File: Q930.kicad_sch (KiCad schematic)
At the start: 2 parts, among them U1 MW-R-WX

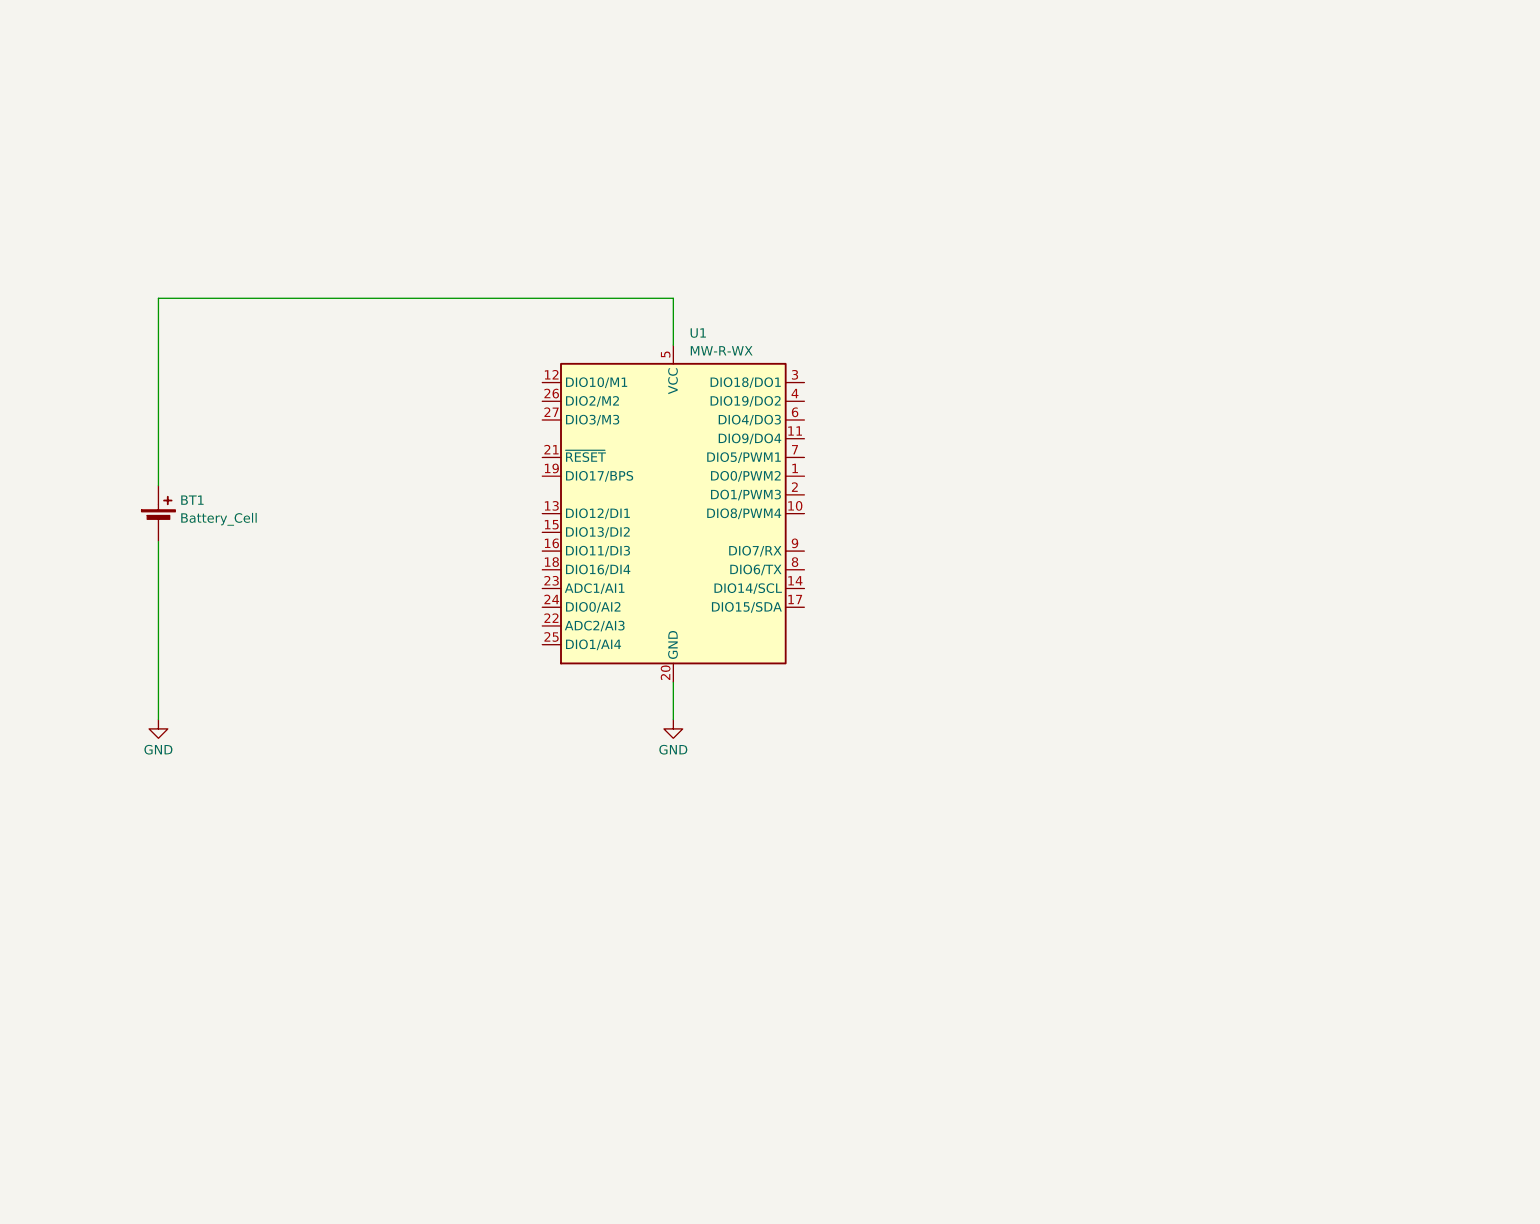
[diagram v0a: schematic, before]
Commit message: continue
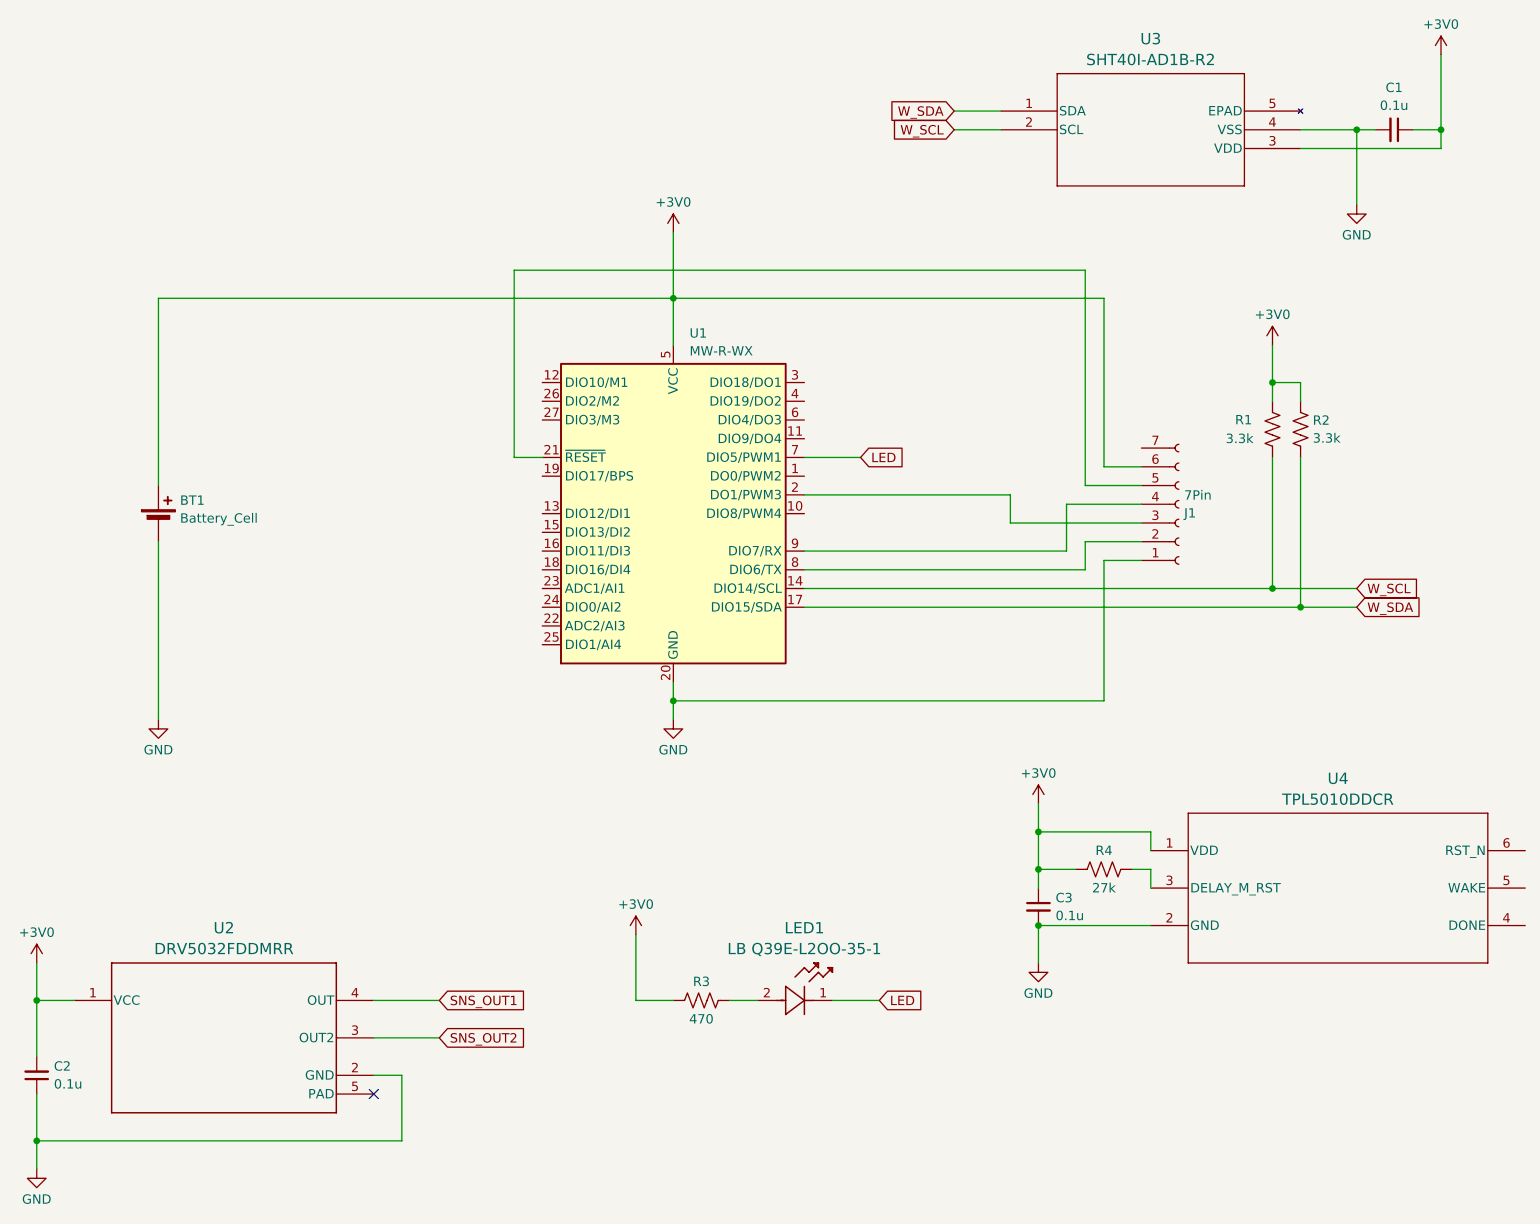
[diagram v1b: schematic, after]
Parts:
- added C1, C2, C3: 0.1u, symbol Device:C_Small
- added J1: 7Pin, symbol Connector:Conn_01x07_Socket
- added LED1: LB Q39E-L2OO-35-1, LED_LBQ39E_OSR, symbol q930:LB_Q39E-L2OO-35-1
- added R1, R2: 3.3k, symbol Device:R_US
- added R3: 470, symbol Device:R_US
- added R4: 27k, symbol Device:R_US
- added U2: DRV5032FDDMRR, DMR0004A, symbol q930:DRV5032FDDMRR
- added U3: SHT40I-AD1B-R2, SHT40I_SEN, symbol q930:SHT40I-AD1B-R2
- added U4: TPL5010DDCR, DDC0006A_N, symbol q930:TPL5010DDCR
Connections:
- net GND: now also C1.2, C2.1, C3.2, J1.1 (Pin_1), U2.2 (GND), U3.4 (VSS), U4.2 (GND)
- net +3V0: now reaches BT1.1 (+), U1.5 (VCC)
- net +3V0: now also C1.1, C2.2, C3.1, J1.6 (Pin_6), R1.1, R2.1, R3.1, R4.1, U2.1 (VCC), U3.3 (VDD), U4.1 (VDD)
- net W_SCL: now reaches U1.14 (DIO14/SCL)
- net W_SCL: now also R1.2, U3.2 (SCL)
- net W_SDA: now reaches U1.17 (DIO15/SDA)
- net W_SDA: now also R2.2, U3.1 (SDA)
- net at U1.2 (DO1/PWM3): now also J1.3 (Pin_3)
- net at U1.21 (~{RESET}): now also J1.5 (Pin_5)
- net LED: now reaches U1.7 (DIO5/PWM1)
- net LED: now also LED1.1
- net at U1.8 (DIO6/TX): now also J1.2 (Pin_2)
- net at U1.9 (DIO7/RX): now also J1.4 (Pin_4)
- new net: LED1.2, R3.2
- new net: R4.2, U4.3 (DELAY_M_RST)
- new net SNS_OUT1: U2.4 (OUT)
- new net SNS_OUT2: U2.3 (OUT2)
- no-connect marks 0 -> 1
